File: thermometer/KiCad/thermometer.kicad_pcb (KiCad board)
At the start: 2 copper layers, 23 x 17 mm, 5 parts, among them J1 Conn_01x06_Pin, U1 DS18B20

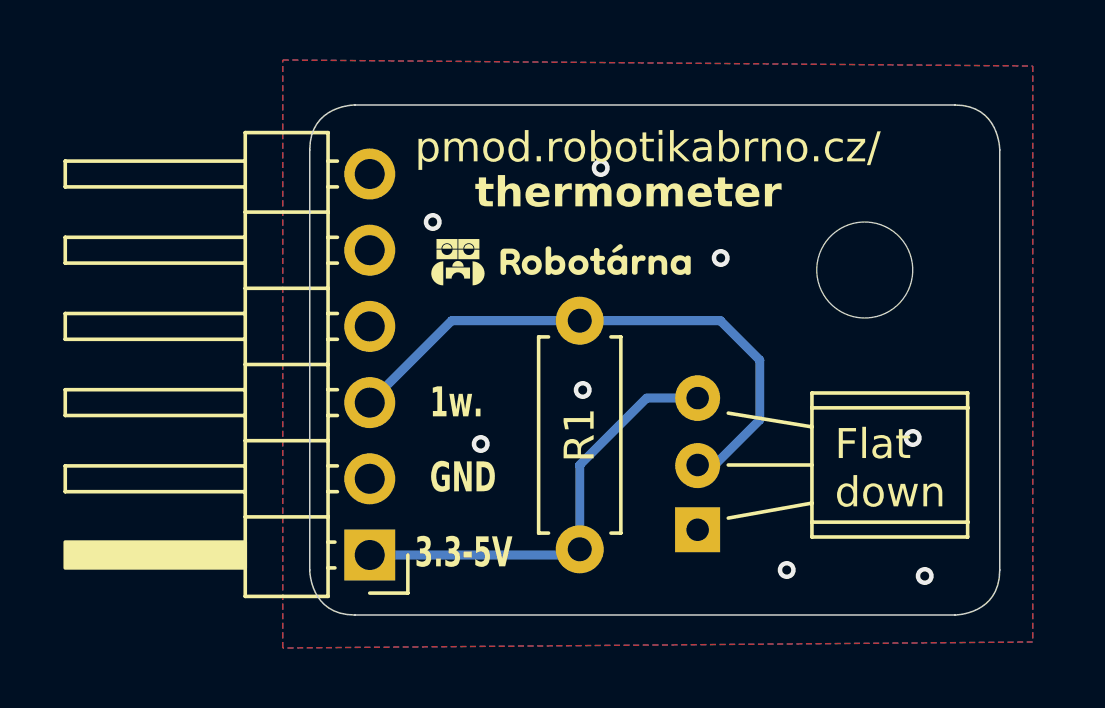
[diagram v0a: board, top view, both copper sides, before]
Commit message: Deployed d972a79 with MkDocs version: 1.6.0
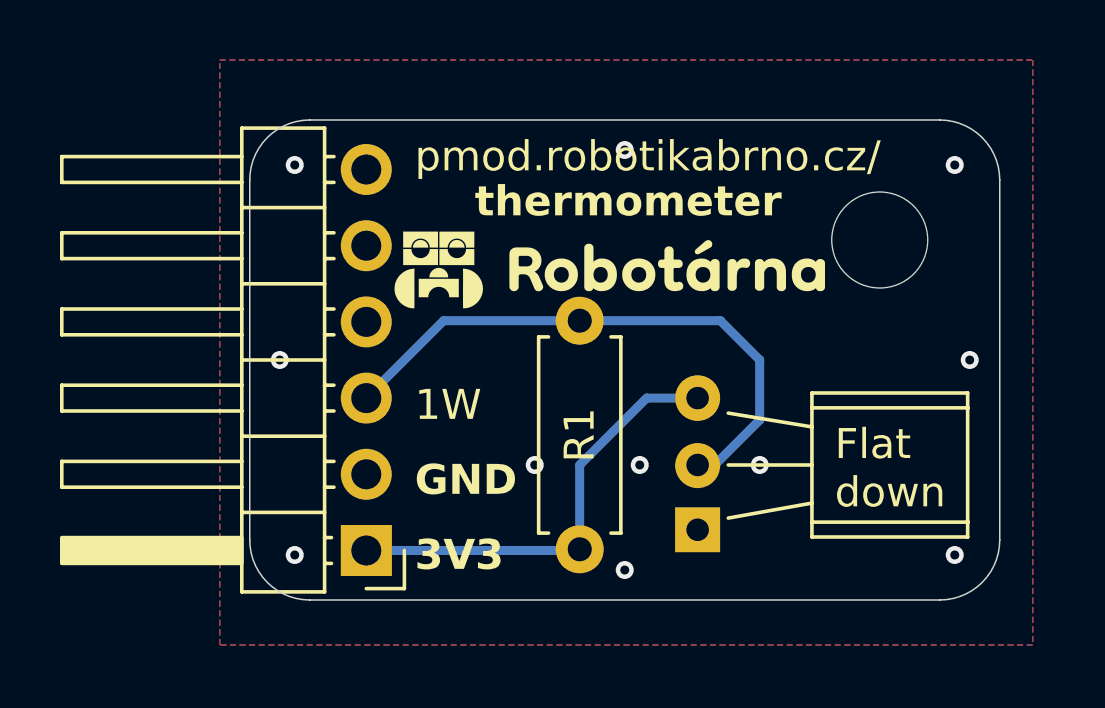
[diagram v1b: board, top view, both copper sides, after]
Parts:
- removed G***: LOGO, LOGO
- moved H1 1.12 mm to (157.5, 106.0)
- moved J1 0.19 mm to (140.4, 116.3)
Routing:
- net GND: vias 8 -> 11
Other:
- board size 23 x 17 mm -> 25 x 16 mm
- board text added: "1W"
- board text added: "36mm"
- board text added: "3V3"
- board text added: "50mm"
- board text removed: "1w."
- board text removed: "3.3-5V"
